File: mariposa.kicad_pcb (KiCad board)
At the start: 4 copper layers, 45 x 100 mm, 93 parts, among them J1 Conn_01x28_MountingPin, J2 Conn_01x03_MountingPin, J3 Conn_ARM_SWD_TagConnect_TC203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, J4 USB_C_Receptacle_USB2.0_16P, J6 Conn_01x10_MountingPin, J8 Conn_01x04_MountingPin, J9 Conn_02x03_Odd_Even, SW1 SW_Push, SW3 SW_Push, U1 TPS62840DLC, U2 BQ25170DSGR, U3 LM66100DCK, U4 TPS22917DBV, U6 LM66100DCK, U7 SN74LV1T125DCK, Y1 CFPX-217 32.768KHz

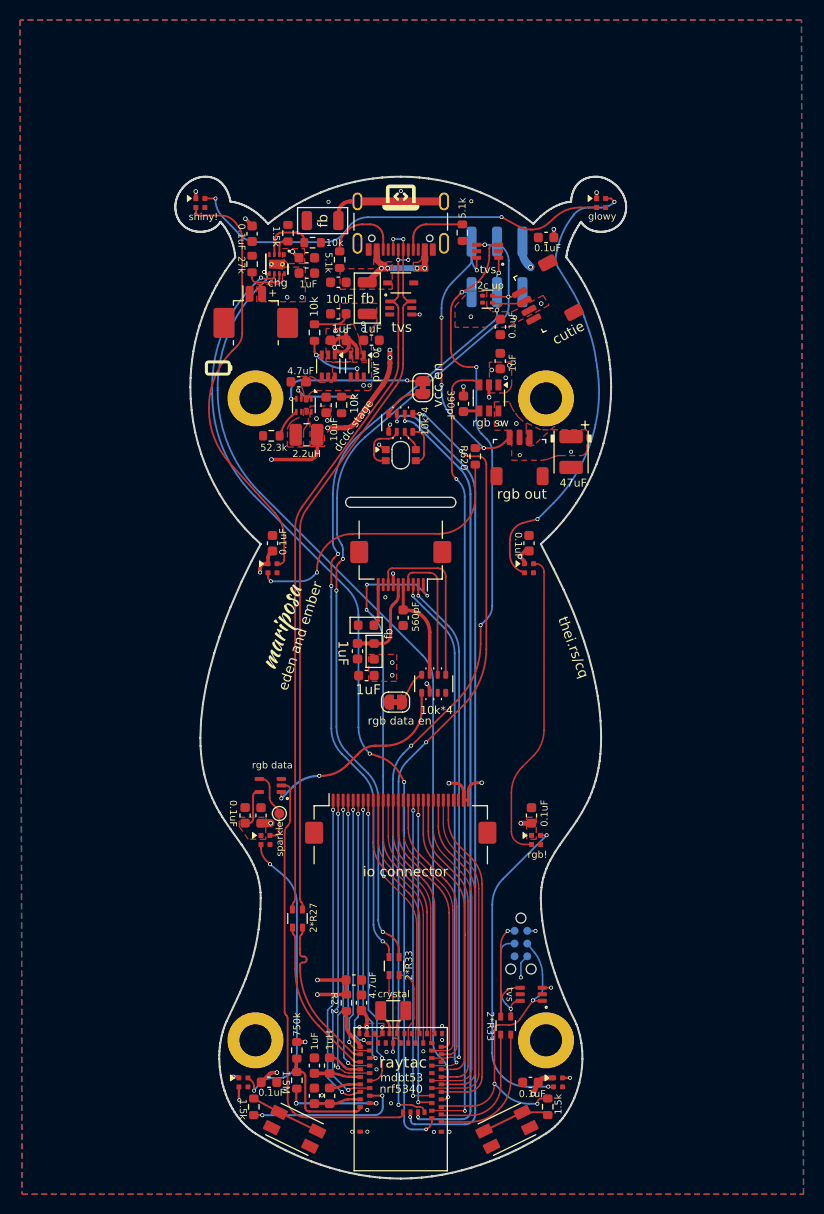
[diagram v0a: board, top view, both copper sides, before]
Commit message: progress
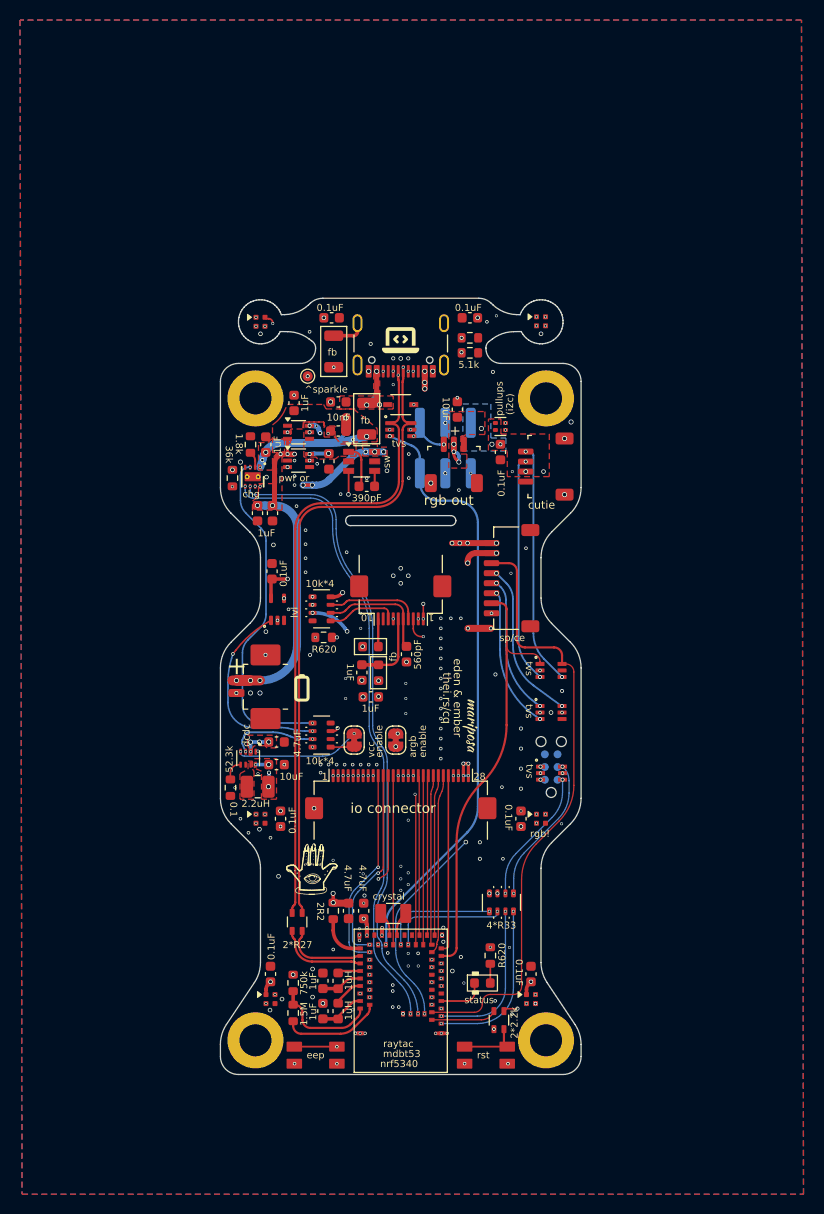
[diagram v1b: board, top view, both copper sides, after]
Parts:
- removed C13: 47uF, PCM_Capacitor_Tantalum_SMD_AKL:CP_EIA-3528-12_Kemet-T
- removed C22, C23: 0.1uF, Capacitor_SMD:C_0603_1608Metric
- removed D21, D22: SK6805-EC14, coquette_footprints:SK6805-EC14
- removed LED1: LED_Generic_RGB_RABG, coquette_footprints:E6CC1205RGBC3UDA
- removed R12, R14, R16: 10k, Resistor_SMD:R_0603_1608Metric
- removed R5, R6: 1.5k, Resistor_SMD:R_0603_1608Metric
- removed RN1, RN2: 2*R33, Resistor_SMD:R_Array_Convex_2x0603
- added C53: 10uF, Capacitor_SMD:C_0603_1608Metric, F.Cu at (153.2, 66.8)
- added D1: LED, PCM_LED_SMD_AKL:LED_0603_1608Metric, F.Cu at (155.7, 124.0)
- added D14: TPD4E1U06, coquette_footprints:TPD4E1U06, F.Cu at (162.5, 97.0)
- added J5: Conn_01x08_MountingPin, Connector_JST:JST_SH_SM08B-SRSS-TB_1x08-1MP_P1.00mm_Horizontal, F.Cu at (158.6, 83.6)
- added R8: R620, Resistor_SMD:R_0603_1608Metric, F.Cu at (156.4, 121.3)
- added RN8: R33*4, PCM_Resistor_SMD_AKL:R_Array_Convex_4x0603, F.Cu at (157.6, 116.0)
- added RN9: 2*2.2k, Resistor_SMD:R_Array_Convex_2x0603, F.Cu at (157.3, 127.7)
- R15: value 27k -> 36k
- R7: value 1.5k -> 1.8k
- moved D16 81.6 mm to (161.5, 58.0)
- moved C17 73.5 mm to (160.5, 123.1), turned to -90 degrees
- moved D20 70.2 mm to (133.5, 107.6)
- moved C16 64.3 mm to (159.5, 107.6)
- moved C15 53.9 mm to (154.4, 57.6), turned to 0 degrees
- moved D15 51.7 mm to (133.5, 58.0)
- moved C14 50.4 mm to (140.6, 57.6), turned to 180 degrees
- moved D19 50.1 mm to (134.5, 125.6)
- moved TP5 43.7 mm to (138.2, 63.5)
- moved D12 42.3 mm to (162.5, 92.8), turned to 0 degrees
- moved BT1 36.8 mm to (133.5, 94.5), turned to 90 degrees
- moved C21 36.3 mm to (135.5, 107.6), turned to 90 degrees
- moved C45 36.2 mm to (135.1, 102.2), turned to 0 degrees
- moved C44 36.0 mm to (135.1, 100.0), turned to 0 degrees
- moved JP2 35.8 mm to (142.8, 99.8)
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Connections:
- D10 pad 3: unconnected-(D10-L2-Pad3) -> gpio2
- D10 pad 4: VCC -> argb_data_out
- D12 pad 1: sda -> sp/ce pwm
- D12 pad 3: gpio2 -> sda
- D12 pad 6: argb_data_out -> sp/ce cs
- MDBT1 pad 10: ch24 -> unconnected-(MDBT1-P1.06-Pad10)
- MDBT1 pad 11: ch23 -> unconnected-(MDBT1-P1.04-Pad11)
- MDBT1 pad 12: ch22 -> ch14
- MDBT1 pad 13: ch21 -> ch15
- MDBT1 pad 14: ch20 -> ch16
- MDBT1 pad 16: ch19 -> ch17
- MDBT1 pad 2: Net-(MDBT1-SWDCLK) -> swdclk_nrf
- MDBT1 pad 20: ch16 -> sp/ce pwm
- MDBT1 pad 21: ch15 -> ch23
- MDBT1 pad 22: ch14 -> ch24
- MDBT1 pad 23: ch12 -> ch21
- MDBT1 pad 25: ch13 -> ch22
- MDBT1 pad 26: ch11 -> ch20
- MDBT1 pad 27: ch10 -> ch19
- MDBT1 pad 28: ch9 -> ch18
- MDBT1 pad 3: chg_pg -> eepy
- MDBT1 pad 31: Net-(MDBT1-P1.03/TWI) -> scl_nrf
- MDBT1 pad 33: Net-(MDBT1-P1.02/TWI) -> sda_nrf
- MDBT1 pad 35: gpio2 -> ch13
- MDBT1 pad 37: unconnected-(MDBT1-P0.04/AIN0-Pad37) -> gpio2
- MDBT1 pad 39: unconnected-(MDBT1-P0.05/AIN1-Pad39) -> ch12
- MDBT1 pad 4: Net-(MDBT1-SWDIO) -> swdio_nrf
- MDBT1 pad 43: ch6 -> ch11
- MDBT1 pad 45: ch5 -> ch10
- MDBT1 pad 47: ch7 -> ch9
- MDBT1 pad 49: ch4 -> ch8
- MDBT1 pad 5: ext_on -> sp/ce cs
- MDBT1 pad 51: ch3 -> ch7
- MDBT1 pad 53: ch8 -> ch6
- MDBT1 pad 55: ch2 -> ch5
- MDBT1 pad 56: ch1 -> ch4
- MDBT1 pad 57: eepy -> ch3
- MDBT1 pad 62: status_led_blue -> ext_on
- MDBT1 pad 63: status_led_green -> chg_pg
- MDBT1 pad 64: status_led_red -> chg_stat
- MDBT1 pad 7: ch18 -> ch1
- MDBT1 pad 8: chg_stat -> status_led
- MDBT1 pad 9: ch17 -> ch2
- R13 pad 2: Net-(D22-DOUT) -> Net-(D20-DOUT)
- RN6 pad 1: VDC -> vcc_en
- RN6 pad 2: stat_blue -> GND
- RN6 pad 3: stat_red -> ll_pull_down
- RN6 pad 4: stat_green -> GND
- RN6 pad 5: status_led_blue -> bat_ts
- RN6 pad 6: status_led_green -> ll_oe
- RN6 pad 7: status_led_red -> vcc_mode
- RN6 pad 8: vcc_en -> VDC
- RN7 pad 2: extcomin -> disp
- RN7 pad 3: disp -> extcomin
- RN7 pad 4: ll_pull_down -> VBUS
- RN7 pad 5: ll_oe -> USB_ST
- RN7 pad 6: VCC -> GND
- RN7 pad 7: GND -> VCC
- U1 pad 3: Net-(U1-MODE) -> vcc_mode
- U2 pad 3: Net-(U2-TS) -> bat_ts
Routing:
- net PRI_LO: track 248.3 -> 33.7 mm, vias 15 -> 20
- net status_led_red: track 82.8 -> 0.00 mm, vias 2 -> 0
- net status_led_blue: track 79.4 -> 0.00 mm, vias 4 -> 0
- net status_led_green: track 78.9 -> 0.00 mm, vias 2 -> 0
- net sp/ce cs: track 0.00 -> 60.7 mm
- net VDC: track 7.81 -> 64.7 mm, vias 7 -> 14
- net miso: track 0.00 -> 49.0 mm, vias 0 -> 3
- net sp/ce pwm: track 0.00 -> 43.9 mm
- net Net-(D21-DOUT): track 42.9 -> 0.00 mm
- net chg_pg: track 98.6 -> 62.5 mm, vias 4 -> 2
- net bat_ts: track 0.00 -> 34.0 mm, vias 0 -> 2
- net gpio2: track 90.4 -> 59.0 mm, vias 5 -> 2
- net chg_stat: track 93.6 -> 62.5 mm
- net GND: track 7.27 -> 38.0 mm, vias 21 -> 183
- net Net-(D22-DOUT): track 29.0 -> 0.00 mm, vias 2 -> 0
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- added copper zone on In3.Cu, net GND
- added copper zone on In4.Cu, net GND
- added copper zone on In2.Cu, net LINE
- added copper zone on B.Cu, net VCC
- added copper zone on In3.Cu, net VCC
- added copper zone on In3.Cu, net VDC
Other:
- board size 45 x 100 mm -> 36 x 77.5 mm
- copper layers 4 -> 6
- board text added: "(i2c)"
- board text added: "0.1"
- board text added: "1"
- board text added: "1.8k"
- board text added: "10"
- board text added: "2*2.2k"
- board text added: "28"
- board text added: "2R2"
- board text added: "36k"
- board text added: "4*R33"
- board text added: "^sparkle"
- board text added: "add-on"
- board text added: "argb"
- board text added: "dcdc"
- board text added: "eden & ember"
- board text added: "eep"
- board text added: "enable"
- board text added: "lvl"
- board text added: "pullups"
- board text added: "rst"
- board text added: "sp/ce"
- board text added: "status"
- board text added: "sw"
- board text added: "vcc"
- board text removed: "1.5k"
- board text removed: "10k"
- board text removed: "2*R33"
- board text removed: "27k"
- board text removed: "47uF"
- board text removed: "R2.2"
- board text removed: "dcdc stage"
- board text removed: "eden and ember"
- board text removed: "glowy"
- board text removed: "i2c up"
- board text removed: "rgb data"
- board text removed: "rgb data en"
- board text removed: "rgb sw"
- board text removed: "shiny!"
- board text removed: "sparkle"
- board text removed: "vcc en"
